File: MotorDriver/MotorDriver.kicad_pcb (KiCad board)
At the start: 2 copper layers, 70 x 70 mm, 77 parts, among them J1 Conn_01x01, J2 Conn_01x01, J3 Conn_01x01, J4 Conn_01x01, J5 Conn_02x04_Odd_Even, J6 Conn_02x03_Odd_Even, J7 4P4C, J8 4P4C, Q1 Q_NMOS_GDS, Q2 Q_NMOS_GDS, Q3 Q_NMOS_GSD, SW1 SW_Push, SW2 SW_SPDT, SW3 SW_Push, U1 FAN7190, U2 ACS712xLCTR-20A, U3 MAX485E, U4 STM32F103C8Tx, U5 LD1117S50TR_SOT223, U6 MCP1700-3302E_SOT23, Y1 8Mhz

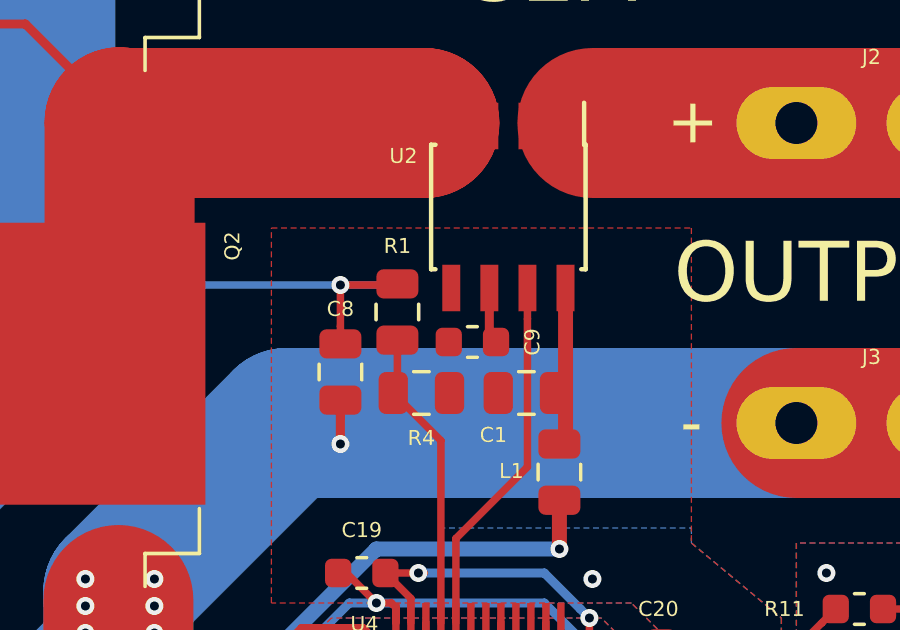
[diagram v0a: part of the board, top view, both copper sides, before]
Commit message: Minor changes.
Squashed commit of the following:

commit b4817053897282ec246551fcbd580ae102a3b469
Author: Paweł <mackipawel@gmail.com>
Date:   Thu Apr 25 22:57:44 2019 +0200

    Minor changes.
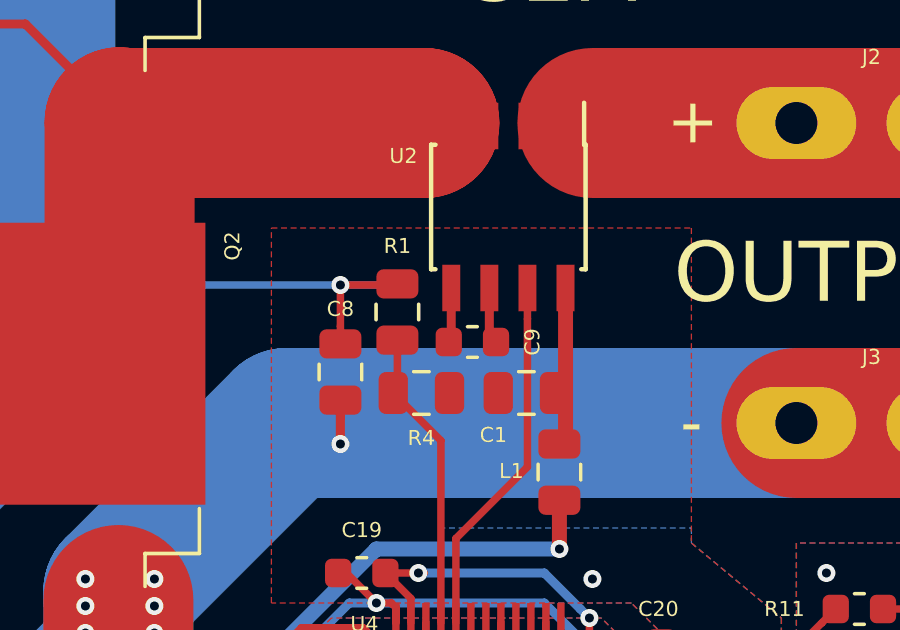
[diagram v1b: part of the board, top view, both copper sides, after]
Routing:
- net GNDA: track 12.2 -> 14.1 mm
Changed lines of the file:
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@@
     (thickness 1.6)
     (drawings 18)
-    (tracks 609)
+    (tracks 611)
     (zones 0)
     (modules 77)
@@
   )
   (setup
-    (last_trace_width 0.25)
+    (last_trace_width 0.3)
     (user_trace_width 0.3)
     (user_trace_width 0.5)
@@
   (segment (start 160 113.25) (end 160.95 113.25) (width 0.5) (layer F.Cu) (net 6))
   (via (at 155.2 100.2) (size 0.6) (drill 0.3) (layers F.Cu B.Cu) (net 6))
+  (segment (start 150.495 92.2175) (end 150.4125 92.3) (width 0.3) (layer F.Cu) (net 6))
+  (segment (start 150.495 90.5) (end 150.495 92.2175) (width 0.3) (layer F.Cu) (net 6))
   (segment (start 128.6375 92.1) (end 128.6375 94) (width 0.3) (layer F.Cu) (net 7) (status 30))
   (segment (start 133.51 102.175) (end 134.36 102.175) (width 0.3) (layer F.Cu) (net 7))
@@
     (connect_pads (clearance 0.25))
     (min_thickness 0.25)
-    (fill yes (arc_segments 16) (thermal_gap 0.5) (thermal_bridge_width 0.5))
+    (fill yes (arc_segments 16) (thermal_gap 0.3) (thermal_bridge_width 0.4))
     (polygon
       (pts
@@
     (connect_pads (clearance 0.25))
     (min_thickness 0.25)
-    (fill yes (arc_segments 16) (thermal_gap 0.5) (thermal_bridge_width 0.5))
+    (fill yes (arc_segments 16) (thermal_gap 0.3) (thermal_bridge_width 0.4))
     (polygon
       (pts
@@
     (connect_pads (clearance 0.25))
     (min_thickness 0.25)
-    (fill yes (arc_segments 16) (thermal_gap 0.5) (thermal_bridge_width 0.5))
+    (fill yes (arc_segments 16) (thermal_gap 0.3) (thermal_bridge_width 0.4))
     (polygon
       (pts
@@
     (connect_pads (clearance 0.25))
     (min_thickness 0.25)
-    (fill yes (arc_segments 16) (thermal_gap 0.5) (thermal_bridge_width 0.5))
+    (fill yes (arc_segments 16) (thermal_gap 0.3) (thermal_bridge_width 0.4))
     (polygon
       (pts
